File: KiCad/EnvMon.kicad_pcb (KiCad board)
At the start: 2 copper layers, 44.5 x 37 mm, 17 parts, among them J1 USB-C, J2 DC, J3 GPIO, M1 D24V5F3-NoSHDN, M2 OLED1.5-RGB, M3 SCD30-4pin, U1 FT230XQ, U2 ESP32-WROOM-32

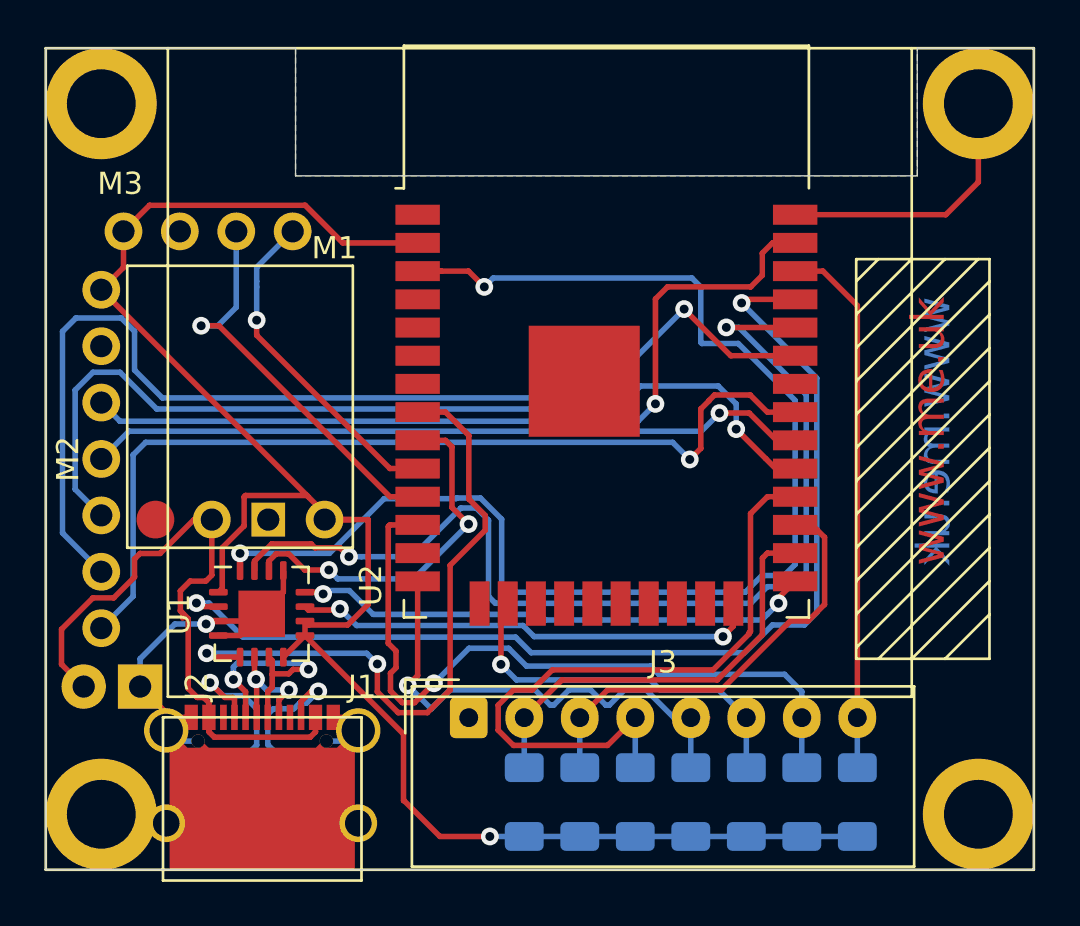
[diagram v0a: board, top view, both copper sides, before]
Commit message: SCAD
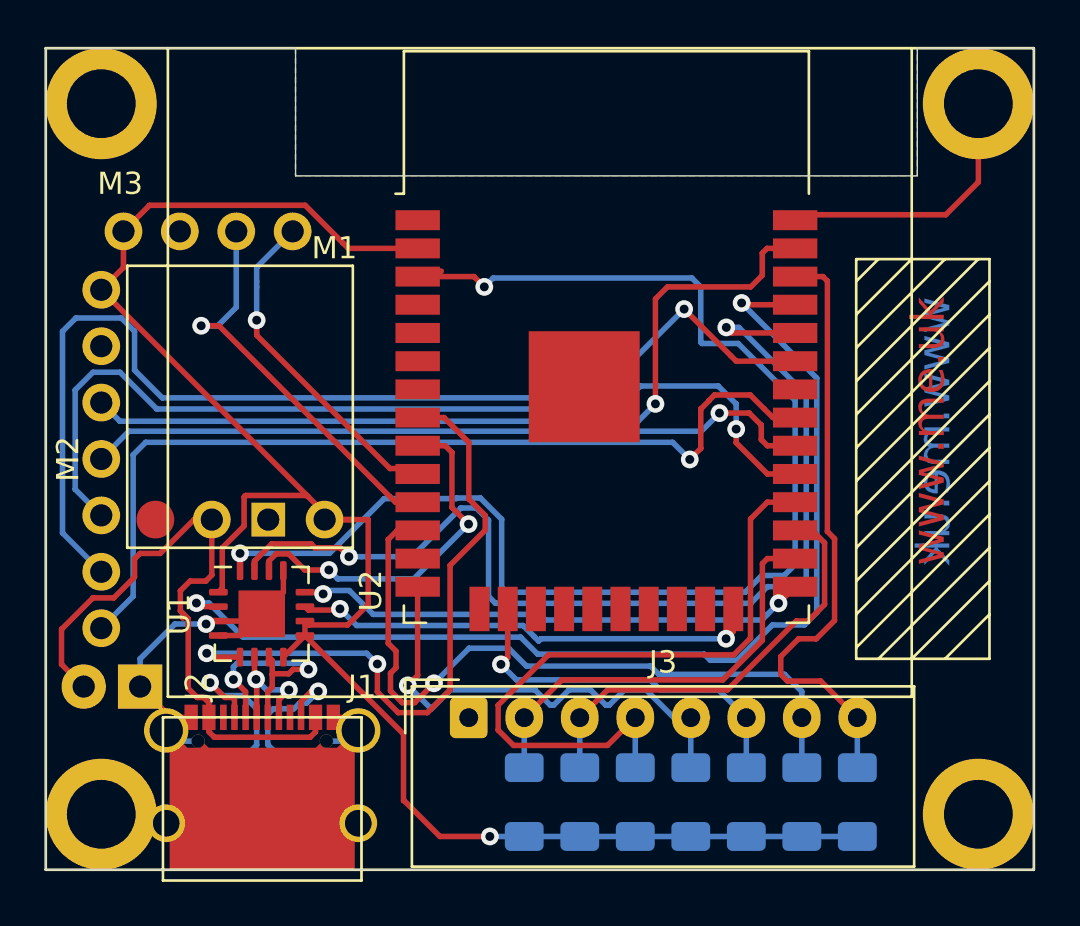
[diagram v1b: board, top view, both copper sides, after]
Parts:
- moved U2 0.25 mm to (115.2, 79.0)
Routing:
- net IO7: track 24.7 -> 27.8 mm
- net CBUS1: track 21.1 -> 23.0 mm
